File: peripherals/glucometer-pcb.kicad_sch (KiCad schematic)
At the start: 12 parts, among them U1 ESP32_DevKit_V1_DOIT

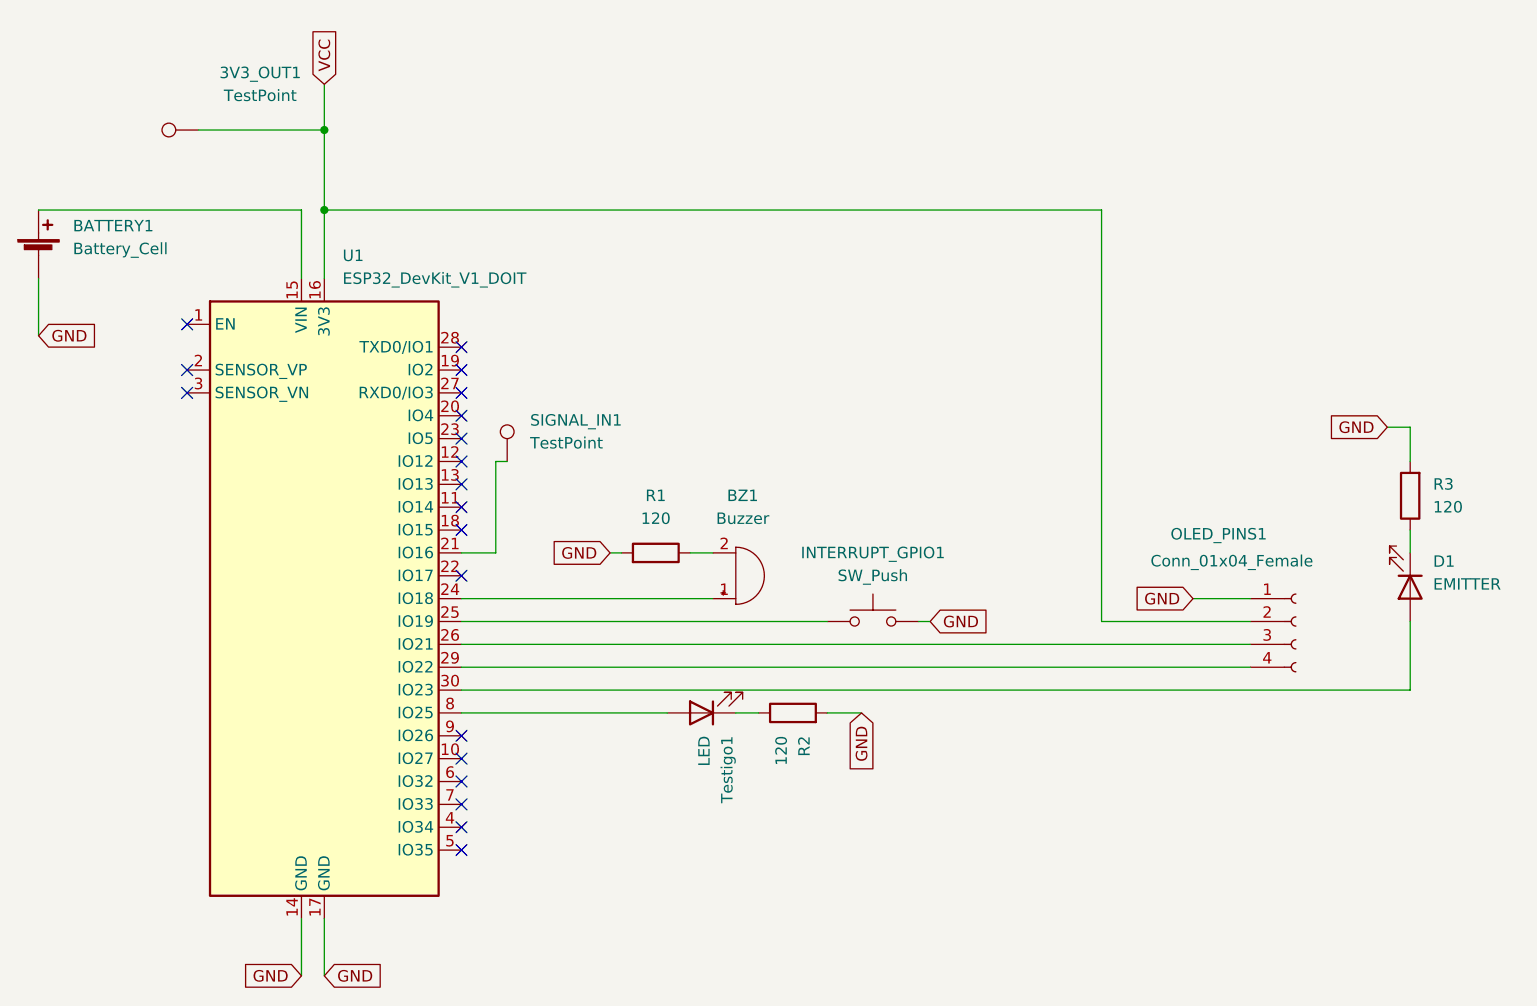
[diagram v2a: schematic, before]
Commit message: last update emmiter pcb
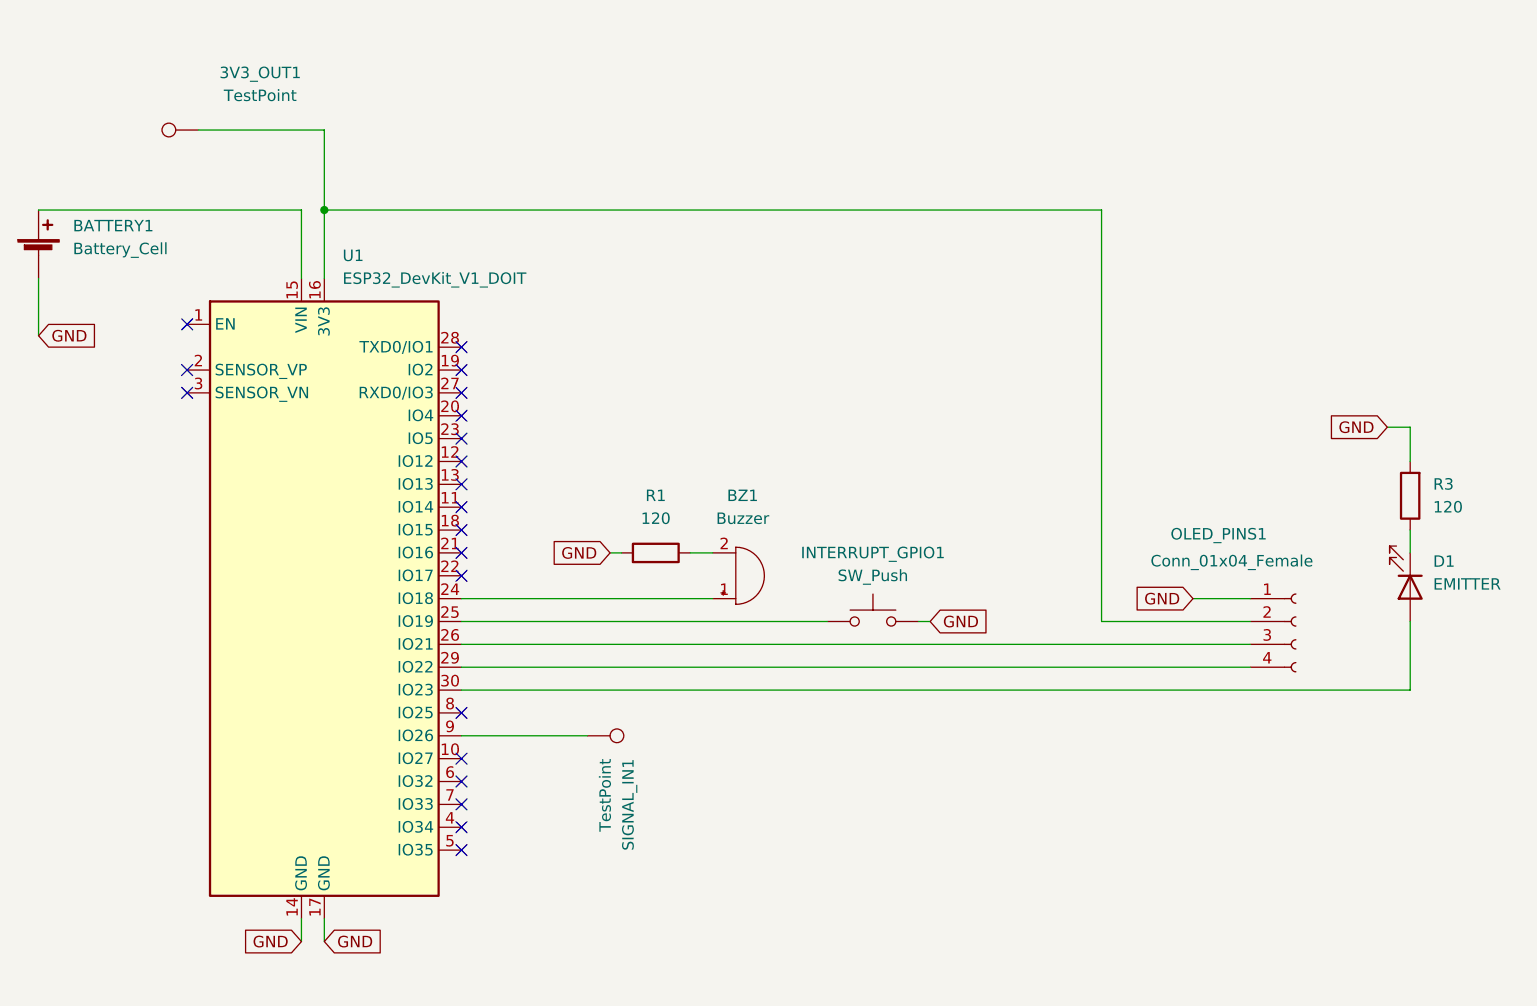
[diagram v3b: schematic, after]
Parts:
- removed R2: 120, Resistor_THT:R_Axial_DIN0204_L3.6mm_D1.6mm_P7.62mm_Horizontal, symbol Device:R
- removed Testigo1: LED, LED_THT:LED_D3.0mm_FlatTop, symbol Device:LED
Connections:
- net at SIGNAL_IN1.1: now also U1.9 (IO26); no longer U1.21 (IO16)
- net VCC: no longer names the net of 3V3_OUT1.1, OLED_PINS1.2 (Pin_2), U1.16 (3V3)
- no-connect marks 19 -> 20
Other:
- moved on the sheet: SIGNAL_IN1
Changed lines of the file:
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@@
 (kicad_sch (version 20211123) (generator eeschema)
   (paper "A4")
-  (junction (at 68.58 39.37) (diameter 0) (color 0 0 0 0)
-  )
   (junction (at 68.58 48.26) (diameter 0) (color 0 0 0 0)
   )
@@
   (no_connect (at 83.82 63.5))
   (no_connect (at 83.82 109.22))
-  (no_connect (at 83.82 114.3))
   (no_connect (at 83.82 116.84))
   (no_connect (at 83.82 111.76))
@@
   (no_connect (at 83.82 83.82))
   (no_connect (at 83.82 66.04))
-  (no_connect (at 83.82 106.68))
-  (wire (pts (xy 83.82 104.14) (xy 106.68 104.14))
-    (stroke (width 0) (type default) (color 0 0 0 0))
-  )
-  (wire (pts (xy 87.63 86.36) (xy 87.63 76.2))
+  (no_connect (at 83.82 104.14))
+  (no_connect (at 83.82 114.3))
+  (no_connect (at 83.82 86.36))
+  (wire (pts (xy 83.82 106.68) (xy 97.79 106.68))
     (stroke (width 0) (type default) (color 0 0 0 0))
   )
@@
     (stroke (width 0) (type default) (color 0 0 0 0))
   )
-  (wire (pts (xy 68.58 127) (xy 68.58 133.35))
-    (stroke (width 0) (type default) (color 0 0 0 0))
-  )
   (wire (pts (xy 83.82 99.06) (xy 171.45 99.06))
     (stroke (width 0) (type default) (color 0 0 0 0))
@@
     (stroke (width 0) (type default) (color 0 0 0 0))
   )
-  (wire (pts (xy 66.04 127) (xy 66.04 133.35))
-    (stroke (width 0) (type default) (color 0 0 0 0))
-  )
   (wire (pts (xy 154.94 93.98) (xy 154.94 48.26))
     (stroke (width 0) (type default) (color 0 0 0 0))
@@
     (stroke (width 0) (type default) (color 0 0 0 0))
   )
-  (wire (pts (xy 83.82 86.36) (xy 87.63 86.36))
-    (stroke (width 0) (type default) (color 0 0 0 0))
-  )
   (wire (pts (xy 66.04 48.26) (xy 66.04 55.88))
     (stroke (width 0) (type default) (color 0 0 0 0))
   )
-  (wire (pts (xy 68.58 34.29) (xy 68.58 39.37))
-    (stroke (width 0) (type default) (color 0 0 0 0))
-  )
   (wire (pts (xy 83.82 91.44) (xy 111.76 91.44))
     (stroke (width 0) (type default) (color 0 0 0 0))
   )
-  (wire (pts (xy 128.27 104.14) (xy 124.46 104.14))
-    (stroke (width 0) (type default) (color 0 0 0 0))
-  )
   (wire (pts (xy 83.82 96.52) (xy 171.45 96.52))
     (stroke (width 0) (type default) (color 0 0 0 0))
@@
     (stroke (width 0) (type default) (color 0 0 0 0))
   )
+  (wire (pts (xy 66.04 127) (xy 66.04 129.54))
+    (stroke (width 0) (type default) (color 0 0 0 0))
+  )
   (wire (pts (xy 109.22 86.36) (xy 111.76 86.36))
     (stroke (width 0) (type default) (color 0 0 0 0))
@@
     (stroke (width 0) (type default) (color 0 0 0 0))
   )
-  (wire (pts (xy 87.63 76.2) (xy 88.9 76.2))
-    (stroke (width 0) (type default) (color 0 0 0 0))
-  )
   (wire (pts (xy 134.62 93.98) (xy 135.89 93.98))
     (stroke (width 0) (type default) (color 0 0 0 0))
@@
     (stroke (width 0) (type default) (color 0 0 0 0))
   )
-  (wire (pts (xy 116.84 104.14) (xy 114.3 104.14))
+  (wire (pts (xy 68.58 127) (xy 68.58 129.54))
     (stroke (width 0) (type default) (color 0 0 0 0))
   )
@@
     )
   )
+  (global_label "GND" (shape input) (at 68.58 129.54 0) (fields_autoplaced)
+    (effects (font (size 1.27 1.27)) (justify left))
+    (property "Referencias entre hojas" "${INTERSHEET_REFS}" (id 0) (at 74.8636 129.4606 0)
+      (effects (font (size 1.27 1.27)) (justify left) hide)
+    )
+  )
   (global_label "GND" (shape input) (at 100.33 86.36 180) (fields_autoplaced)
     (effects (font (size 1.27 1.27)) (justify right))
@@
     )
   )
-  (global_label "GND" (shape input) (at 68.58 133.35 0) (fields_autoplaced)
-    (effects (font (size 1.27 1.27)) (justify left))
-    (property "Referencias entre hojas" "${INTERSHEET_REFS}" (id 0) (at 74.8636 133.4294 0)
-      (effects (font (size 1.27 1.27)) (justify left) hide)
-    )
-  )
-  (global_label "GND" (shape input) (at 128.27 104.14 270) (fields_autoplaced)
+  (global_label "GND" (shape input) (at 66.04 129.54 180) (fields_autoplaced)
     (effects (font (size 1.27 1.27)) (justify right))
-    (property "Referencias entre hojas" "${INTERSHEET_REFS}" (id 0) (at 128.1906 110.4236 90)
+    (property "Referencias entre hojas" "${INTERSHEET_REFS}" (id 0) (at 59.7564 129.4606 0)
       (effects (font (size 1.27 1.27)) (justify right) hide)
     )
@@
     )
   )
-  (global_label "GND" (shape input) (at 66.04 133.35 180) (fields_autoplaced)
-    (effects (font (size 1.27 1.27)) (justify right))
-    (property "Referencias entre hojas" "${INTERSHEET_REFS}" (id 0) (at 59.7564 133.2706 0)
-      (effects (font (size 1.27 1.27)) (justify right) hide)
-    )
-  )
-  (global_label "VCC" (shape input) (at 68.58 34.29 90) (fields_autoplaced)
-    (effects (font (size 1.27 1.27)) (justify left))
-    (property "Referencias entre hojas" "${INTERSHEET_REFS}" (id 0) (at 68.5006 28.2483 90)
-      (effects (font (size 1.27 1.27)) (justify left) hide)
-    )
-  )
   (global_label "GND" (shape input) (at 135.89 93.98 0) (fields_autoplaced)
     (effects (font (size 1.27 1.27)) (justify left))
-    (property "Referencias entre hojas" "${INTERSHEET_REFS}" (id 0) (at 142.1736 94.0594 0)
+    (property "Referencias entre hojas" "${INTERSHEET_REFS}" (id 0) (at 142.1736 93.9006 0)
       (effects (font (size 1.27 1.27)) (justify left) hide)
     )
-  )
-  (symbol (lib_id "Device:LED") (at 110.49 104.14 180) (unit 1)
-    (in_bom yes) (on_board yes)
-    (property "Reference" "Testigo1" (id 0) (at 113.3476 106.68 90)
-      (effects (font (size 1.27 1.27)) (justify left))
-    )
-    (property "Value" "LED" (id 1) (at 110.8076 106.68 90)
-      (effects (font (size 1.27 1.27)) (justify left))
-    )
-    (property "Footprint" "LED_THT:LED_D3.0mm_FlatTop" (id 2) (at 110.49 104.14 0)
-      (effects (font (size 1.27 1.27)) hide)
-    )
-    (property "Datasheet" "~" (id 3) (at 110.49 104.14 0)
-      (effects (font (size 1.27 1.27)) hide)
-    )
-    (pin "1")
-    (pin "2")
   )
   (symbol (lib_id "Connector:Conn_01x04_Female") (at 176.53 93.98 0) (unit 1)
@@
     (pin "2")
   )
-  (symbol (lib_id "Connector:TestPoint") (at 88.9 76.2 0) (mirror y) (unit 1)
-    (in_bom yes) (on_board yes) (fields_autoplaced)
-    (property "Reference" "SIGNAL_IN1" (id 0) (at 91.44 71.6279 0)
+  (symbol (lib_id "Connector:TestPoint") (at 97.79 106.68 270) (mirror x) (unit 1)
+    (in_bom yes) (on_board yes) (fields_autoplaced)
+    (property "Reference" "SIGNAL_IN1" (id 0) (at 102.3621 109.22 0)
       (effects (font (size 1.27 1.27)) (justify right))
     )
-    (property "Value" "TestPoint" (id 1) (at 91.44 74.1679 0)
+    (property "Value" "TestPoint" (id 1) (at 99.8221 109.22 0)
       (effects (font (size 1.27 1.27)) (justify right))
     )
-    (property "Footprint" "TestPoint:TestPoint_Keystone_5015_Micro-Minature" (id 2) (at 83.82 76.2 0)
-      (effects (font (size 1.27 1.27)) hide)
-    )
-    (property "Datasheet" "~" (id 3) (at 83.82 76.2 0)
+    (property "Footprint" "TestPoint:TestPoint_Keystone_5015_Micro-Minature" (id 2) (at 97.79 101.6 0)
+      (effects (font (size 1.27 1.27)) hide)
+    )
+    (property "Datasheet" "~" (id 3) (at 97.79 101.6 0)
       (effects (font (size 1.27 1.27)) hide)
     )
@@
     )
     (property "Datasheet" "~" (id 3) (at 129.54 88.9 0)
-      (effects (font (size 1.27 1.27)) hide)
-    )
-    (pin "1")
-    (pin "2")
-  )
-  (symbol (lib_id "Device:R") (at 120.65 104.14 90) (unit 1)
-    (in_bom yes) (on_board yes) (fields_autoplaced)
-    (property "Reference" "R2" (id 0) (at 121.9201 106.68 0)
-      (effects (font (size 1.27 1.27)) (justify right))
-    )
-    (property "Value" "120" (id 1) (at 119.3801 106.68 0)
-      (effects (font (size 1.27 1.27)) (justify right))
-    )
-    (property "Footprint" "Resistor_THT:R_Axial_DIN0204_L3.6mm_D1.6mm_P7.62mm_Horizontal" (id 2) (at 120.65 105.918 90)
-      (effects (font (size 1.27 1.27)) hide)
-    )
-    (property "Datasheet" "~" (id 3) (at 120.65 104.14 0)
       (effects (font (size 1.27 1.27)) hide)
     )
@@
       (reference "R1") (unit 1) (value "120") (footprint "Resistor_THT:R_Axial_DIN0204_L3.6mm_D1.6mm_P7.62mm_Horizontal")
     )
-    (path "/b6a30bc2-0d74-43ed-aa2b-a3d443bd9193"
-      (reference "R2") (unit 1) (value "120") (footprint "Resistor_THT:R_Axial_DIN0204_L3.6mm_D1.6mm_P7.62mm_Horizontal")
-    )
     (path "/48716155-f70c-423a-8030-4a2d322cc6d9"
       (reference "R3") (unit 1) (value "120") (footprint "Resistor_THT:R_Axial_DIN0204_L3.6mm_D1.6mm_P7.62mm_Horizontal")
@@
       (reference "SIGNAL_IN1") (unit 1) (value "TestPoint") (footprint "TestPoint:TestPoint_Keystone_5015_Micro-Minature")
     )
-    (path "/019be3e5-53d3-4756-bc1c-bd7873df24c4"
-      (reference "Testigo1") (unit 1) (value "LED") (footprint "LED_THT:LED_D3.0mm_FlatTop")
-    )
     (path "/d6ca7d44-4b9c-4d66-afa6-a65a2e89d1cd"
